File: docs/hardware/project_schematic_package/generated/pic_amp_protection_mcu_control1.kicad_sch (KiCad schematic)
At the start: 9 parts, among them J3 LCD_I2C, Q1 Q_NMOS, U1 PIC16F18855-xSO

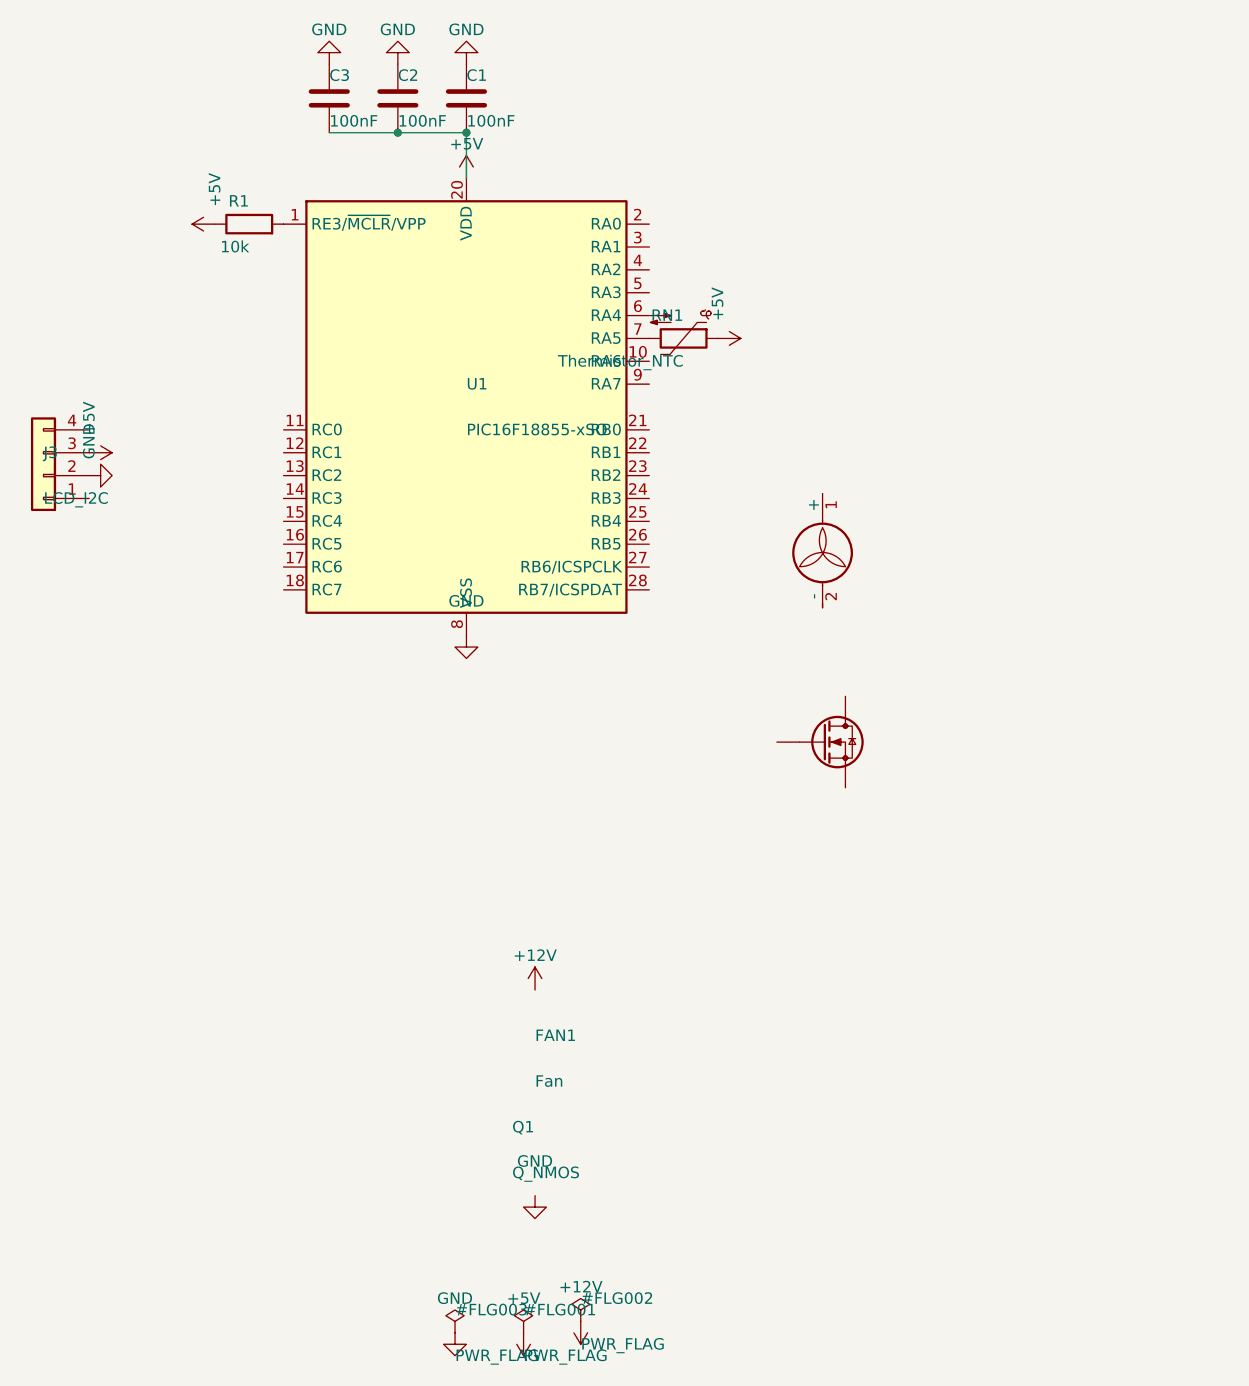
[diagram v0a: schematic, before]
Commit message: Update schematic generation work
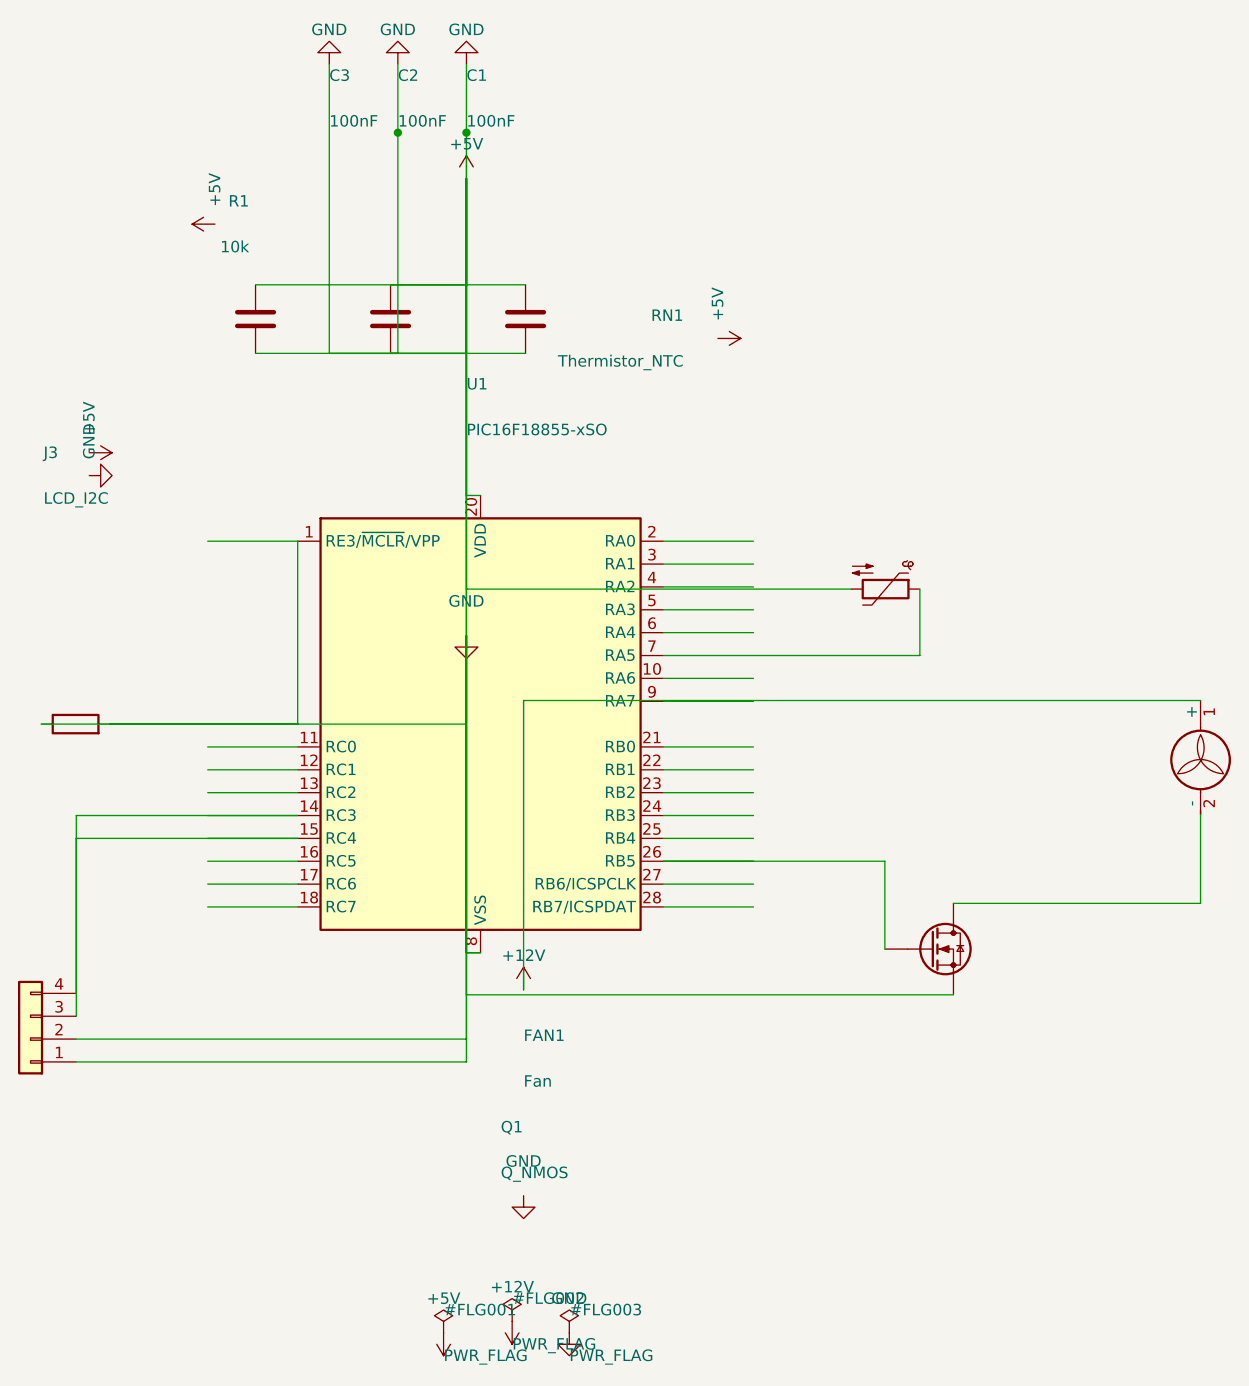
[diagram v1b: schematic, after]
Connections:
- net GND is gone; now on net +5V: C1.1, C2.1, C3.1, J3.2 (Pin_2), U1.19 (VSS), U1.8 (VSS)
- net +12V: now also FAN1.1 (+)
- net +5V: now also J3.1 (Pin_1), Q1.S, R1.2, RN1.2, U1.1 (RE3/~{MCLR}/VPP); no longer J3.3 (Pin_3), RN1.1
- net at J3.4 (Pin_4): now also J3.3 (Pin_3), U1.14 (RC3), U1.15 (RC4)
- net at U1.26 (RB5): now also Q1.G
- net at U1.7 (RA5): now also RN1.1; no longer RN1.2
- net at FAN1.2 (-): now also Q1.D
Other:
- moved on the sheet: C1, C2, C3, FAN1, J3, Q1, R1, RN1, U1
